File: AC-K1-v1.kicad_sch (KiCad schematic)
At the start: 3 parts, among them U1 nice_nano

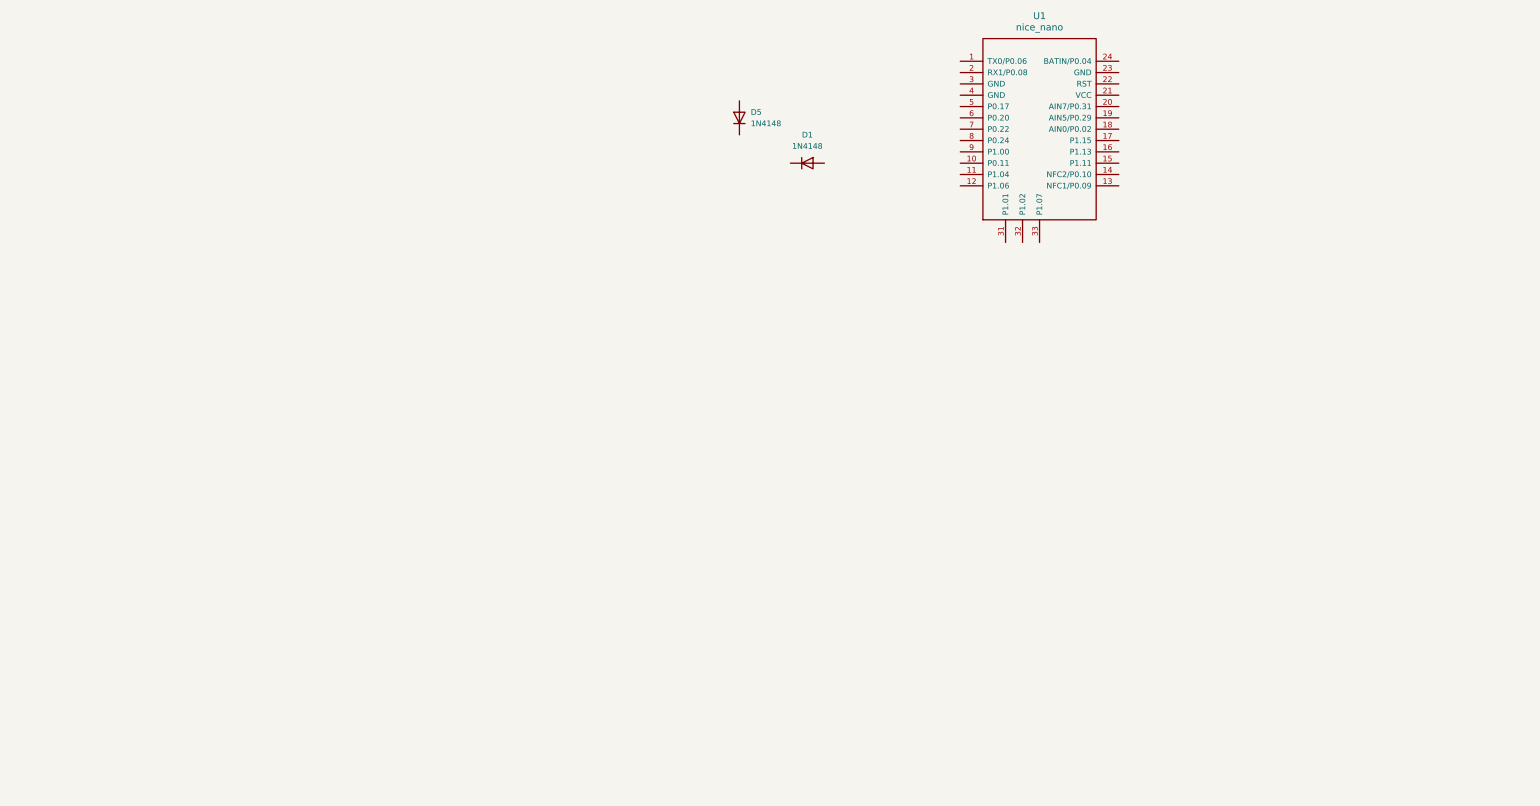
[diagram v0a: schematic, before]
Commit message: Worked on spreadsheet
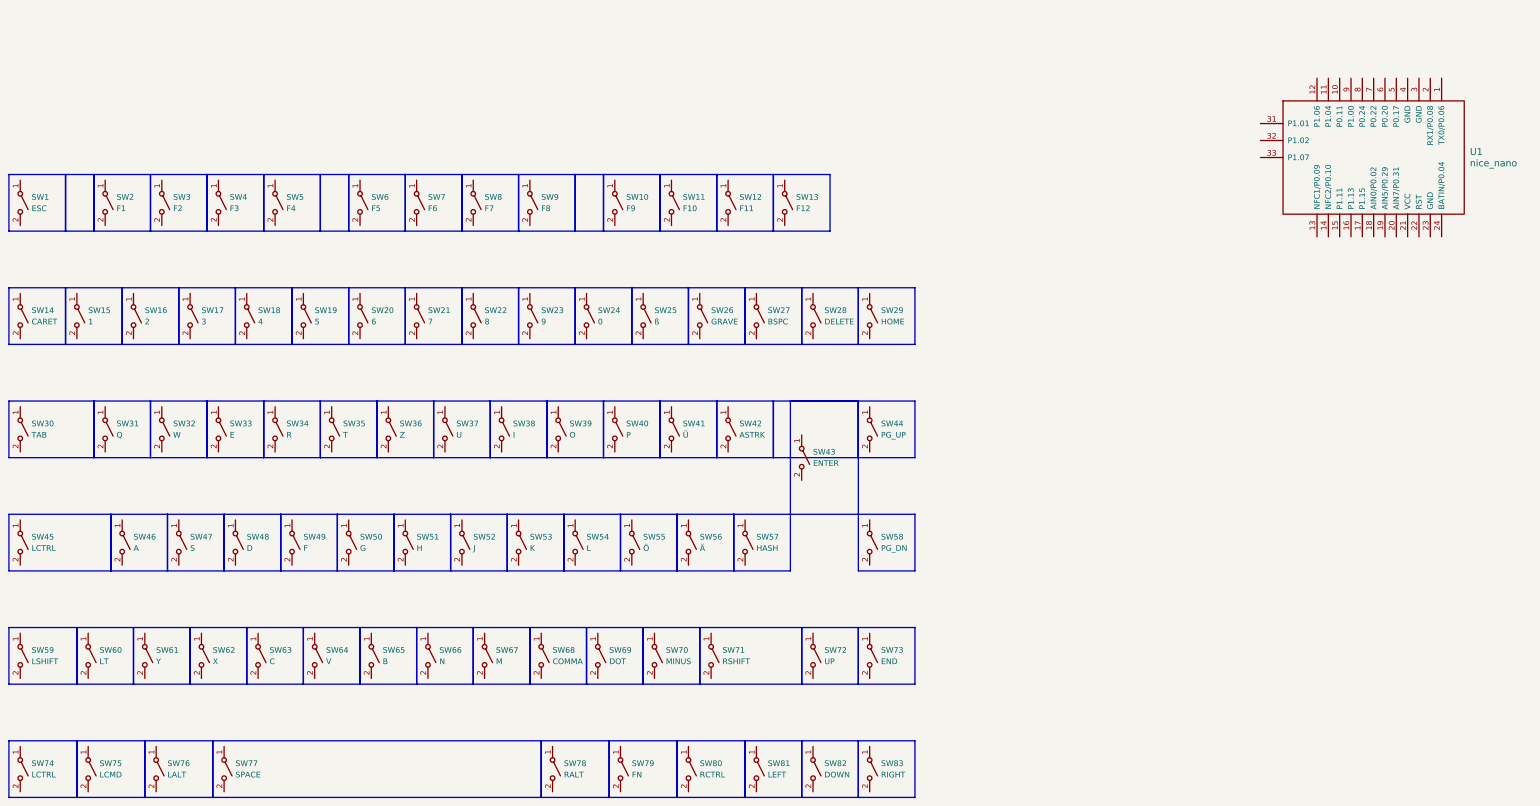
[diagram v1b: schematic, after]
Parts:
- removed D1, D5: 1N4148, Diode_THT:D_DO-35_SOD27_P7.62mm_Horizontal, symbol Diode:1N4148
- added SW1: ESC, Switch_Keyboard_Kailh:SW_Kailh_Choc_V1V2_1.00u, symbol Switch:SW_SPST
- added SW10: F9, Switch_Keyboard_Kailh:SW_Kailh_Choc_V1V2_1.00u, symbol Switch:SW_SPST
- added SW11: F10, Switch_Keyboard_Kailh:SW_Kailh_Choc_V1V2_1.00u, symbol Switch:SW_SPST
- added SW12: F11, Switch_Keyboard_Kailh:SW_Kailh_Choc_V1V2_1.00u, symbol Switch:SW_SPST
- added SW13: F12, Switch_Keyboard_Kailh:SW_Kailh_Choc_V1V2_1.00u, symbol Switch:SW_SPST
- added SW14: CARET, Switch_Keyboard_Kailh:SW_Kailh_Choc_V1V2_1.00u, symbol Switch:SW_SPST
- added SW15: 1, Switch_Keyboard_Kailh:SW_Kailh_Choc_V1V2_1.00u, symbol Switch:SW_SPST
- added SW16: 2, Switch_Keyboard_Kailh:SW_Kailh_Choc_V1V2_1.00u, symbol Switch:SW_SPST
- added SW17: 3, Switch_Keyboard_Kailh:SW_Kailh_Choc_V1V2_1.00u, symbol Switch:SW_SPST
- added SW18: 4, Switch_Keyboard_Kailh:SW_Kailh_Choc_V1V2_1.00u, symbol Switch:SW_SPST
- added SW19: 5, Switch_Keyboard_Kailh:SW_Kailh_Choc_V1V2_1.00u, symbol Switch:SW_SPST
- added SW2: F1, Switch_Keyboard_Kailh:SW_Kailh_Choc_V1V2_1.00u, symbol Switch:SW_SPST
- added SW20: 6, Switch_Keyboard_Kailh:SW_Kailh_Choc_V1V2_1.00u, symbol Switch:SW_SPST
- added SW21: 7, Switch_Keyboard_Kailh:SW_Kailh_Choc_V1V2_1.00u, symbol Switch:SW_SPST
- added SW22: 8, Switch_Keyboard_Kailh:SW_Kailh_Choc_V1V2_1.00u, symbol Switch:SW_SPST
- added SW23: 9, Switch_Keyboard_Kailh:SW_Kailh_Choc_V1V2_1.00u, symbol Switch:SW_SPST
- added SW24: 0, Switch_Keyboard_Kailh:SW_Kailh_Choc_V1V2_1.00u, symbol Switch:SW_SPST
- added SW25: ß, Switch_Keyboard_Kailh:SW_Kailh_Choc_V1V2_1.00u, symbol Switch:SW_SPST
- added SW26: GRAVE, Switch_Keyboard_Kailh:SW_Kailh_Choc_V1V2_1.00u, symbol Switch:SW_SPST
- added SW27: BSPC, Switch_Keyboard_Kailh:SW_Kailh_Choc_V1V2_1.00u, symbol Switch:SW_SPST
- added SW28: DELETE, Switch_Keyboard_Kailh:SW_Kailh_Choc_V1V2_1.00u, symbol Switch:SW_SPST
- added SW29: HOME, Switch_Keyboard_Kailh:SW_Kailh_Choc_V1V2_1.00u, symbol Switch:SW_SPST
- added SW3: F2, Switch_Keyboard_Kailh:SW_Kailh_Choc_V1V2_1.00u, symbol Switch:SW_SPST
- added SW30: TAB, Switch_Keyboard_Kailh:SW_Kailh_Choc_V1V2_1.50u, symbol Switch:SW_SPST
- added SW31: Q, Switch_Keyboard_Kailh:SW_Kailh_Choc_V1V2_1.00u, symbol Switch:SW_SPST
- added SW32: W, Switch_Keyboard_Kailh:SW_Kailh_Choc_V1V2_1.00u, symbol Switch:SW_SPST
- added SW33: E, Switch_Keyboard_Kailh:SW_Kailh_Choc_V1V2_1.00u, symbol Switch:SW_SPST
- added SW34: R, Switch_Keyboard_Kailh:SW_Kailh_Choc_V1V2_1.00u, symbol Switch:SW_SPST
- added SW35: T, Switch_Keyboard_Kailh:SW_Kailh_Choc_V1V2_1.00u, symbol Switch:SW_SPST
- added SW36: Z, Switch_Keyboard_Kailh:SW_Kailh_Choc_V1V2_1.00u, symbol Switch:SW_SPST
- added SW37: U, Switch_Keyboard_Kailh:SW_Kailh_Choc_V1V2_1.00u, symbol Switch:SW_SPST
- added SW38: I, Switch_Keyboard_Kailh:SW_Kailh_Choc_V1V2_1.00u, symbol Switch:SW_SPST
- added SW39: O, Switch_Keyboard_Kailh:SW_Kailh_Choc_V1V2_1.00u, symbol Switch:SW_SPST
- added SW4: F3, Switch_Keyboard_Kailh:SW_Kailh_Choc_V1V2_1.00u, symbol Switch:SW_SPST
- added SW40: P, Switch_Keyboard_Kailh:SW_Kailh_Choc_V1V2_1.00u, symbol Switch:SW_SPST
- added SW41: Ü, Switch_Keyboard_Kailh:SW_Kailh_Choc_V1V2_1.00u, symbol Switch:SW_SPST
- added SW42: ASTRK, Switch_Keyboard_Kailh:SW_Kailh_Choc_V1V2_1.00u, symbol Switch:SW_SPST
- added SW43: ENTER, Switch_Keyboard_Kailh:SW_Kailh_Choc_V1V2_ISOEnter, symbol Switch:SW_SPST
- added SW44: PG_UP, Switch_Keyboard_Kailh:SW_Kailh_Choc_V1V2_1.00u, symbol Switch:SW_SPST
- added SW45: LCTRL, Switch_Keyboard_Kailh:SW_Kailh_Choc_V1V2_1.75u, symbol Switch:SW_SPST
- added SW46: A, Switch_Keyboard_Kailh:SW_Kailh_Choc_V1V2_1.00u, symbol Switch:SW_SPST
- added SW47: S, Switch_Keyboard_Kailh:SW_Kailh_Choc_V1V2_1.00u, symbol Switch:SW_SPST
- added SW48: D, Switch_Keyboard_Kailh:SW_Kailh_Choc_V1V2_1.00u, symbol Switch:SW_SPST
- added SW49: F, Switch_Keyboard_Kailh:SW_Kailh_Choc_V1V2_1.00u, symbol Switch:SW_SPST
- added SW5: F4, Switch_Keyboard_Kailh:SW_Kailh_Choc_V1V2_1.00u, symbol Switch:SW_SPST
- added SW50: G, Switch_Keyboard_Kailh:SW_Kailh_Choc_V1V2_1.00u, symbol Switch:SW_SPST
- added SW51: H, Switch_Keyboard_Kailh:SW_Kailh_Choc_V1V2_1.00u, symbol Switch:SW_SPST
- added SW52: J, Switch_Keyboard_Kailh:SW_Kailh_Choc_V1V2_1.00u, symbol Switch:SW_SPST
- added SW53: K, Switch_Keyboard_Kailh:SW_Kailh_Choc_V1V2_1.00u, symbol Switch:SW_SPST
- added SW54: L, Switch_Keyboard_Kailh:SW_Kailh_Choc_V1V2_1.00u, symbol Switch:SW_SPST
- added SW55: Ö, Switch_Keyboard_Kailh:SW_Kailh_Choc_V1V2_1.00u, symbol Switch:SW_SPST
- added SW56: Ä, Switch_Keyboard_Kailh:SW_Kailh_Choc_V1V2_1.00u, symbol Switch:SW_SPST
- added SW57: HASH, Switch_Keyboard_Kailh:SW_Kailh_Choc_V1V2_1.00u, symbol Switch:SW_SPST
- added SW58: PG_DN, Switch_Keyboard_Kailh:SW_Kailh_Choc_V1V2_1.00u, symbol Switch:SW_SPST
- added SW59: LSHIFT, Switch_Keyboard_Kailh:SW_Kailh_Choc_V1V2_1.25u, symbol Switch:SW_SPST
- added SW6: F5, Switch_Keyboard_Kailh:SW_Kailh_Choc_V1V2_1.00u, symbol Switch:SW_SPST
- added SW60: LT, Switch_Keyboard_Kailh:SW_Kailh_Choc_V1V2_1.00u, symbol Switch:SW_SPST
- added SW61: Y, Switch_Keyboard_Kailh:SW_Kailh_Choc_V1V2_1.00u, symbol Switch:SW_SPST
- added SW62: X, Switch_Keyboard_Kailh:SW_Kailh_Choc_V1V2_1.00u, symbol Switch:SW_SPST
- added SW63: C, Switch_Keyboard_Kailh:SW_Kailh_Choc_V1V2_1.00u, symbol Switch:SW_SPST
- added SW64: V, Switch_Keyboard_Kailh:SW_Kailh_Choc_V1V2_1.00u, symbol Switch:SW_SPST
- added SW65: B, Switch_Keyboard_Kailh:SW_Kailh_Choc_V1V2_1.00u, symbol Switch:SW_SPST
- added SW66: N, Switch_Keyboard_Kailh:SW_Kailh_Choc_V1V2_1.00u, symbol Switch:SW_SPST
- added SW67: M, Switch_Keyboard_Kailh:SW_Kailh_Choc_V1V2_1.00u, symbol Switch:SW_SPST
- added SW68: COMMA, Switch_Keyboard_Kailh:SW_Kailh_Choc_V1V2_1.00u, symbol Switch:SW_SPST
- added SW69: DOT, Switch_Keyboard_Kailh:SW_Kailh_Choc_V1V2_1.00u, symbol Switch:SW_SPST
- added SW7: F6, Switch_Keyboard_Kailh:SW_Kailh_Choc_V1V2_1.00u, symbol Switch:SW_SPST
- added SW70: MINUS, Switch_Keyboard_Kailh:SW_Kailh_Choc_V1V2_1.00u, symbol Switch:SW_SPST
- added SW71: RSHIFT, Switch_Keyboard_Kailh:SW_Kailh_Choc_V1V2_1.75u, symbol Switch:SW_SPST
- added SW72: UP, Switch_Keyboard_Kailh:SW_Kailh_Choc_V1V2_1.00u, symbol Switch:SW_SPST
- added SW73: END, Switch_Keyboard_Kailh:SW_Kailh_Choc_V1V2_1.00u, symbol Switch:SW_SPST
- added SW74: LCTRL, Switch_Keyboard_Kailh:SW_Kailh_Choc_V1V2_1.25u, symbol Switch:SW_SPST
- added SW75: LCMD, Switch_Keyboard_Kailh:SW_Kailh_Choc_V1V2_1.25u, symbol Switch:SW_SPST
- added SW76: LALT, Switch_Keyboard_Kailh:SW_Kailh_Choc_V1V2_1.25u, symbol Switch:SW_SPST
- added SW77: SPACE, Switch_Keyboard_Kailh:SW_Kailh_Choc_V1V2_5.50u, symbol Switch:SW_SPST
- added SW78: RALT, Switch_Keyboard_Kailh:SW_Kailh_Choc_V1V2_1.25u, symbol Switch:SW_SPST
- added SW79: FN, Switch_Keyboard_Kailh:SW_Kailh_Choc_V1V2_1.25u, symbol Switch:SW_SPST
- added SW8: F7, Switch_Keyboard_Kailh:SW_Kailh_Choc_V1V2_1.00u, symbol Switch:SW_SPST
- added SW80: RCTRL, Switch_Keyboard_Kailh:SW_Kailh_Choc_V1V2_1.25u, symbol Switch:SW_SPST
- added SW81: LEFT, Switch_Keyboard_Kailh:SW_Kailh_Choc_V1V2_1.00u, symbol Switch:SW_SPST
- added SW82: DOWN, Switch_Keyboard_Kailh:SW_Kailh_Choc_V1V2_1.00u, symbol Switch:SW_SPST
- added SW83: RIGHT, Switch_Keyboard_Kailh:SW_Kailh_Choc_V1V2_1.00u, symbol Switch:SW_SPST
- added SW9: F8, Switch_Keyboard_Kailh:SW_Kailh_Choc_V1V2_1.00u, symbol Switch:SW_SPST
- U1: footprint (none) -> nice-nano-kicad-master:nice_nano
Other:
- moved on the sheet: U1

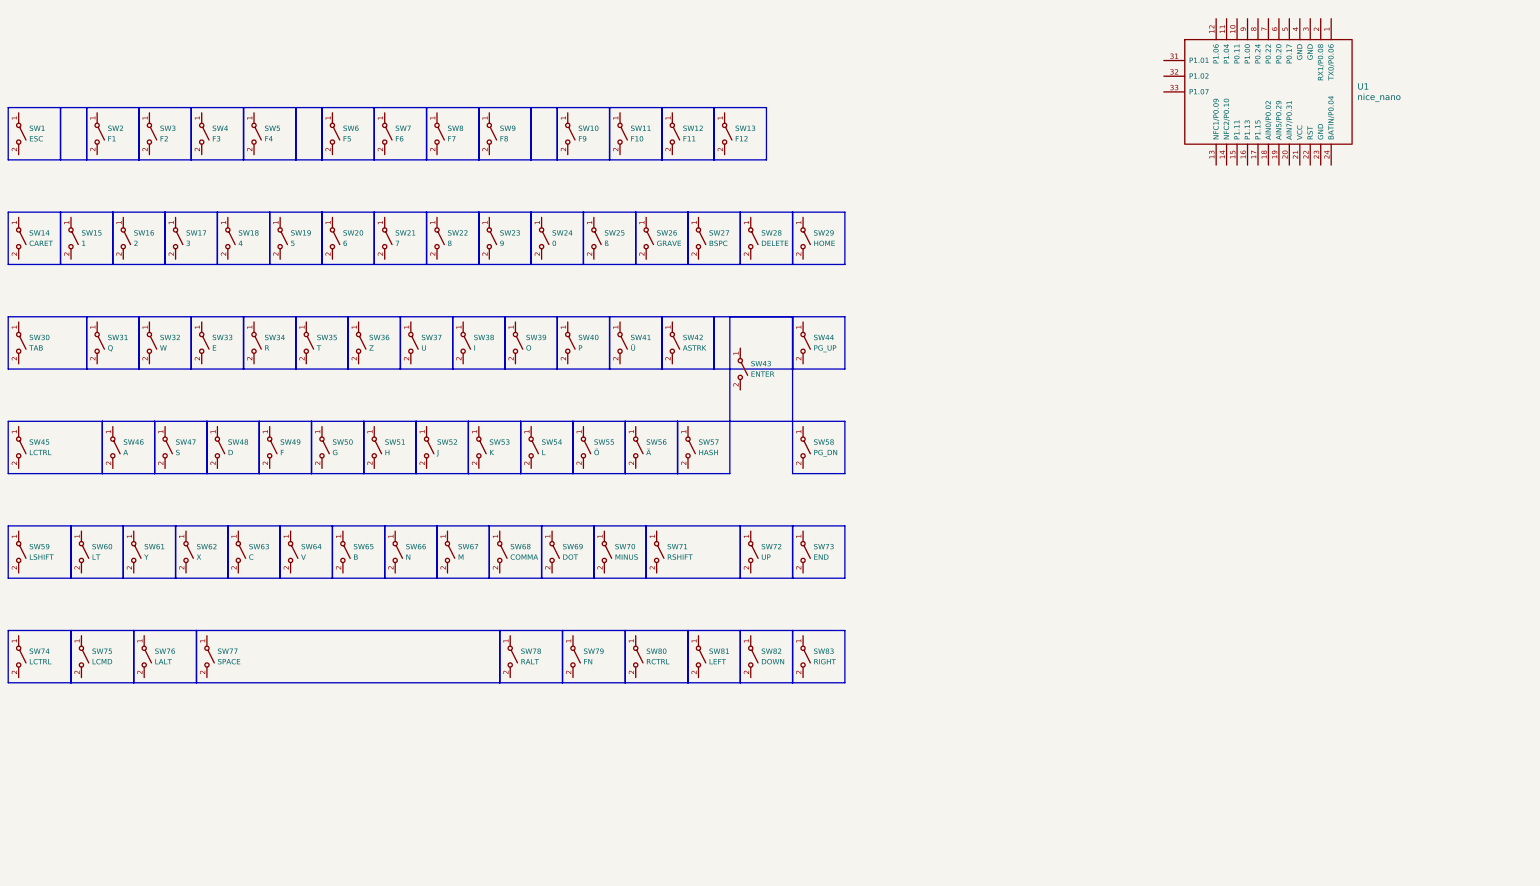
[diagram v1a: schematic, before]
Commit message: Made big part of PCB
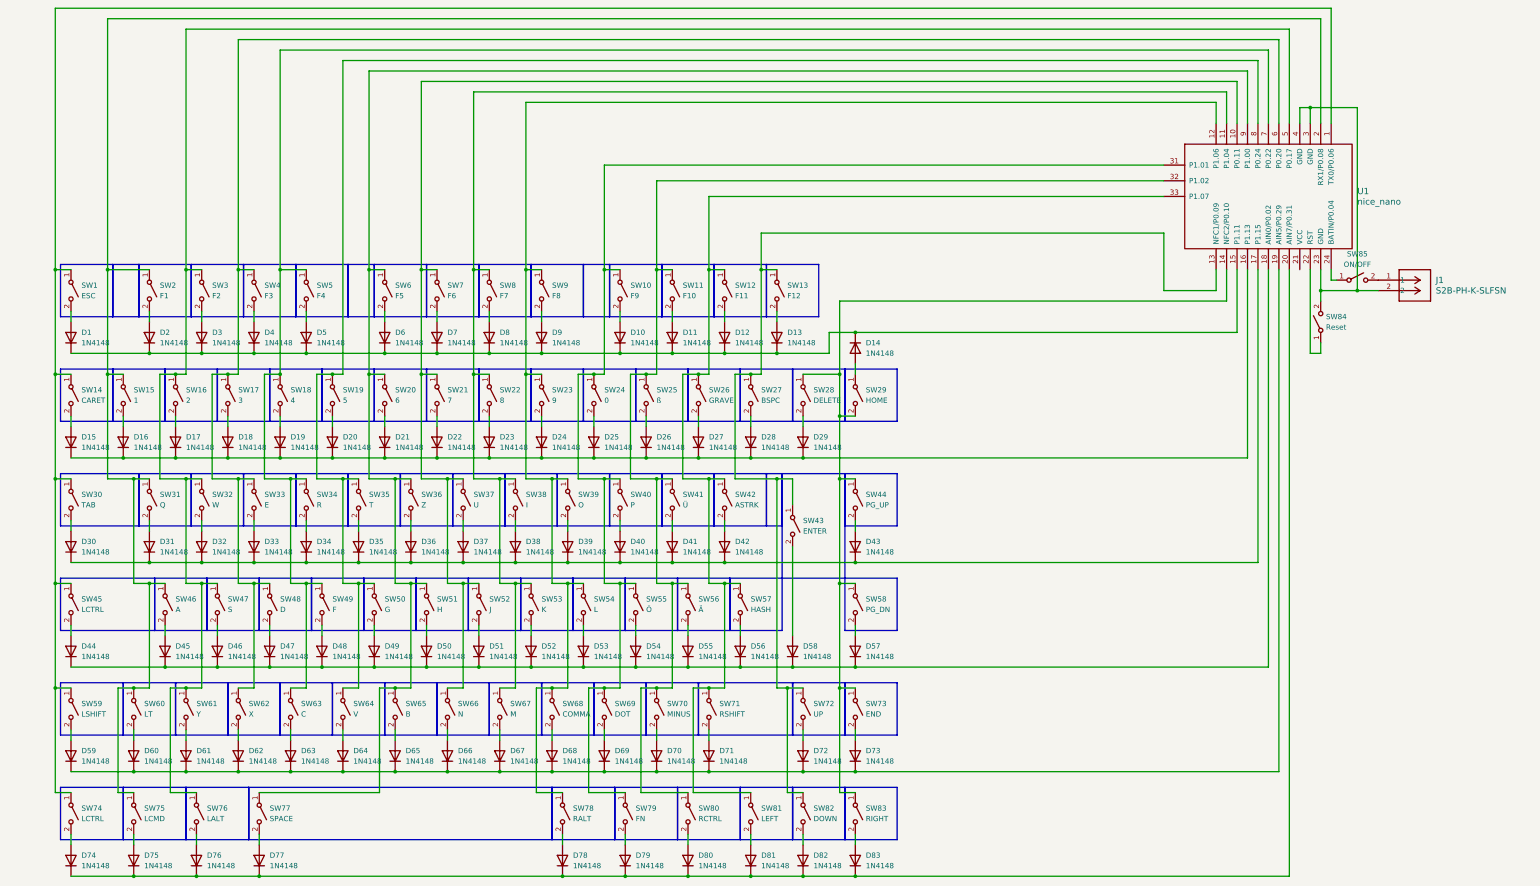
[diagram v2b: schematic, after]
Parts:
- added D1, D10, D11, D12, D13, D14, D15, D16, D17, D18, D19, D2, D20, D21, D22, D23, D24, D25, D26, D27, D28, D29, D3, D30, D31, D32, D33, D34, D35, D36, D37, D38, D39, D4, D40, D41, D42, D43, D44, D45, D46, D47, D48, D49, D5, D50, D51, D52, D53, D54, D55, D56, D57, D58, D59, D6, D60, D61, D62, D63, D64, D65, D66, D67, D68, D69, D7, D70, D71, D72, D73, D74, D75, D76, D77, D78, D79, D8, D80, D81, D82, D83, D9: 1N4148, Diode_THT:D_DO-35_SOD27_P7.62mm_Horizontal, symbol Diode:1N4148
- added J1: S2B-PH-K-SLFSN, Connector_JST:JST_PH_S2B-PH-K_1x02_P2.00mm_Horizontal, symbol 2024-07-08_06-49-09:S2B-PH-K-SLFSN
- added SW84: Reset, Button_Switch_THT:SW_PUSH_1P1T_6x3.5mm_H4.3_APEM_MJTP1243, symbol Switch:SW_SPST
- added SW85: ON/OFF, Switch_Keyboard_Kailh:SW_Kailh_Choc_V1V2_1.00u, symbol Switch:SW_SPST
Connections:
- net at SW31.1 (A): now also SW15.1 (A), SW2.1 (A), SW46.1 (A), SW60.1 (A), SW75.1 (A), U1.2 (RX1/P0.08)
- net at SW31.2 (B): now also D31.2 (A)
- net at SW65.1 (A): now also SW20.1 (A), SW36.1 (A), SW51.1 (A), SW6.1 (A), SW77.1 (A), U1.9 (P1.00)
- net at SW65.2 (B): now also D65.2 (A)
- net at SW8.1 (A): now also SW22.1 (A), SW38.1 (A), SW53.1 (A), SW67.1 (A), U1.11 (P1.04)
- net at SW8.2 (B): now also D8.2 (A)
- net at SW21.1 (A): now also SW37.1 (A), SW52.1 (A), SW66.1 (A), SW7.1 (A), U1.10 (P0.11)
- net at SW21.2 (B): now also D22.2 (A)
- net at SW4.1 (A): now also SW17.1 (A), SW33.1 (A), SW48.1 (A), SW62.1 (A), U1.6 (P0.20)
- net at SW4.2 (B): now also D4.2 (A)
- net at SW28.1 (A): now also SW29.2 (B), SW44.1 (A), SW58.1 (A), SW73.1 (A), SW83.1 (A), U1.14 (NFC2/P0.10)
- net at SW28.2 (B): now also D29.2 (A)
- net at SW2.2 (B): now also D2.2 (A)
- net at SW50.1 (A): now also SW19.1 (A), SW35.1 (A), SW64.1 (A), U1.8 (P0.24)
- net at SW50.2 (B): now also D49.2 (A)
- net at SW13.1 (A): now also SW27.1 (A), SW43.1 (A), SW72.1 (A), SW82.1 (A), U1.13 (NFC1/P0.09)
- net at SW13.2 (B): now also D13.2 (A)
- net at SW12.1 (A): now also SW26.1 (A), SW42.1 (A), SW57.1 (A), SW71.1 (A), SW81.1 (A), U1.33 (P1.07)
- net at SW12.2 (B): now also D12.2 (A)
- net at SW7.2 (B): now also D7.2 (A)
- net at SW44.2 (B): now also D43.2 (A)
- net at SW51.2 (B): now also D50.2 (A)
- net at SW33.2 (B): now also D33.2 (A)
- net at SW62.2 (B): now also D62.2 (A)
- net at SW37.2 (B): now also D37.2 (A)
- net at SW78.1 (A): now also SW23.1 (A), SW39.1 (A), SW54.1 (A), SW68.1 (A), SW9.1 (A), U1.12 (P1.06)
- net at SW78.2 (B): now also D78.2 (A)
- net at SW15.2 (B): now also D16.2 (A)
- net at SW60.2 (B): now also D60.2 (A)
- net at SW42.2 (B): now also D42.2 (A)
- net at SW20.2 (B): now also D21.2 (A)
- net at SW79.1 (A): now also SW10.1 (A), SW24.1 (A), SW40.1 (A), SW55.1 (A), SW69.1 (A), U1.31 (P1.01)
- net at SW79.2 (B): now also D79.2 (A)
- net at SW61.1 (A): now also SW16.1 (A), SW3.1 (A), SW32.1 (A), SW47.1 (A), SW76.1 (A), U1.5 (P0.17)
- net at SW61.2 (B): now also D61.2 (A)
- net at SW6.2 (B): now also D6.2 (A)
- net at SW39.2 (B): now also D39.2 (A)
- net at SW58.2 (B): now also D57.2 (A)
- net at SW32.2 (B): now also D32.2 (A)
- net at SW11.1 (A): now also SW25.1 (A), SW41.1 (A), SW56.1 (A), SW70.1 (A), SW80.1 (A), U1.32 (P1.02)
- net at SW11.2 (B): now also D11.2 (A)
- net at SW55.2 (B): now also D54.2 (A)
- net at SW18.1 (A): now also SW34.1 (A), SW49.1 (A), SW5.1 (A), SW63.1 (A), U1.7 (P0.22)
- net at SW18.2 (B): now also D19.2 (A)
- net at SW71.2 (B): now also D71.2 (A)
- net at SW1.1 (A): now also SW14.1 (A), SW30.1 (A), SW45.1 (A), SW59.1 (A), SW74.1 (A), U1.1 (TX0/P0.06)
- net at SW1.2 (B): now also D1.2 (A)
- net at SW73.2 (B): now also D73.2 (A)
- net at SW83.2 (B): now also D83.2 (A)
- net at SW22.2 (B): now also D23.2 (A)
- net at SW80.2 (B): now also D80.2 (A)
- net at SW25.2 (B): now also D26.2 (A)
- net at SW67.2 (B): now also D67.2 (A)
- net at SW27.2 (B): now also D28.2 (A)
- net at SW53.2 (B): now also D52.2 (A)
- net at U1.15 (P1.11): now also D1.1 (K), D10.1 (K), D11.1 (K), D12.1 (K), D13.1 (K), D14.1 (K), D2.1 (K), D3.1 (K), D4.1 (K), D5.1 (K), D6.1 (K), D7.1 (K), D8.1 (K), D9.1 (K)
- net at U1.16 (P1.13): now also D15.1 (K), D16.1 (K), D17.1 (K), D18.1 (K), D19.1 (K), D20.1 (K), D21.1 (K), D22.1 (K), D23.1 (K), D24.1 (K), D25.1 (K), D26.1 (K), D27.1 (K), D28.1 (K), D29.1 (K)
- net at U1.17 (P1.15): now also D30.1 (K), D31.1 (K), D32.1 (K), D33.1 (K), D34.1 (K), D35.1 (K), D36.1 (K), D37.1 (K), D38.1 (K), D39.1 (K), D40.1 (K), D41.1 (K), D42.1 (K), D43.1 (K)
- net at U1.18 (AIN0/P0.02): now also D44.1 (K), D45.1 (K), D46.1 (K), D47.1 (K), D48.1 (K), D49.1 (K), D50.1 (K), D51.1 (K), D52.1 (K), D53.1 (K), D54.1 (K), D55.1 (K), D56.1 (K), D57.1 (K), D58.1 (K)
- net at U1.19 (AIN5/P0.29): now also D59.1 (K), D60.1 (K), D61.1 (K), D62.1 (K), D63.1 (K), D64.1 (K), D65.1 (K), D66.1 (K), D67.1 (K), D68.1 (K), D69.1 (K), D70.1 (K), D71.1 (K), D72.1 (K), D73.1 (K)
- net at U1.20 (AIN7/P0.31): now also D74.1 (K), D75.1 (K), D76.1 (K), D77.1 (K), D78.1 (K), D79.1 (K), D80.1 (K), D81.1 (K), D82.1 (K), D83.1 (K)
- net at U1.22 (RST): now also SW84.1 (A)
- net at U1.23 (GND): now also U1.3 (GND), U1.4 (GND), J1.2, SW84.2 (B)
- net at U1.24 (BATIN/P0.04): now also SW85.1 (A)
- net at SW75.2 (B): now also D75.2 (A)
- net at SW26.2 (B): now also D27.2 (A)
- net at SW17.2 (B): now also D18.2 (A)
- net at SW66.2 (B): now also D66.2 (A)
- net at SW76.2 (B): now also D76.2 (A)
- net at SW56.2 (B): now also D55.2 (A)
- net at SW16.2 (B): now also D17.2 (A)
- net at SW82.2 (B): now also D82.2 (A)
- net at SW74.2 (B): now also D74.2 (A)
- net at SW68.2 (B): now also D68.2 (A)
- net at SW41.2 (B): now also D41.2 (A)
- net at SW23.2 (B): now also D24.2 (A)
- net at SW59.2 (B): now also D59.2 (A)
- net at SW45.2 (B): now also D44.2 (A)
- net at SW49.2 (B): now also D48.2 (A)
- net at SW30.2 (B): now also D30.2 (A)
- net at SW35.2 (B): now also D35.2 (A)
- net at SW38.2 (B): now also D38.2 (A)
- net at SW48.2 (B): now also D47.2 (A)
- net at SW64.2 (B): now also D64.2 (A)
- net at SW54.2 (B): now also D53.2 (A)
- net at SW72.2 (B): now also D72.2 (A)
- net at SW52.2 (B): now also D51.2 (A)
- net at SW29.1 (A): now also D14.2 (A)
- net at SW19.2 (B): now also D20.2 (A)
- net at SW77.2 (B): now also D77.2 (A)
- net at SW57.2 (B): now also D56.2 (A)
- net at SW3.2 (B): now also D3.2 (A)
- net at SW63.2 (B): now also D63.2 (A)
- net at SW9.2 (B): now also D9.2 (A)
- net at SW40.2 (B): now also D40.2 (A)
- net at SW69.2 (B): now also D69.2 (A)
- net at SW81.2 (B): now also D81.2 (A)
- net at SW14.2 (B): now also D15.2 (A)
- net at SW36.2 (B): now also D36.2 (A)
- net at SW34.2 (B): now also D34.2 (A)
- net at SW10.2 (B): now also D10.2 (A)
- net at SW24.2 (B): now also D25.2 (A)
- net at SW46.2 (B): now also D45.2 (A)
- net at SW43.2 (B): now also D58.2 (A)
- net at SW47.2 (B): now also D46.2 (A)
- net at SW70.2 (B): now also D70.2 (A)
- net at SW5.2 (B): now also D5.2 (A)
- new net: J1.1, SW85.2 (B)
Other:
- moved on the sheet: SW1, SW10, SW11, SW12, SW13, SW14, SW15, SW16, SW17, SW18, SW19, SW2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
